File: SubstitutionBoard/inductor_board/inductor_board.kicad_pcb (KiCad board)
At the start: 2 copper layers, 275.5 x 89.4 mm, 220 parts, among them J1 Conn_Coaxial_Power, J2 Barrel_Jack_Switch, J3 Conn_01x18, J4 Conn_01x06_Socket, K1 FINDER-32.21-x000, K10 FINDER-32.21-x000, K11 FINDER-32.21-x000, K12 FINDER-32.21-x000, K13 FINDER-32.21-x000, K14 FINDER-32.21-x000, K15 FINDER-32.21-x000, K16 FINDER-32.21-x000, K2 FINDER-32.21-x000, K3 FINDER-32.21-x000, K4 FINDER-32.21-x000, K5 FINDER-32.21-x000, K6 FINDER-32.21-x000, K7 FINDER-32.21-x000, K8 FINDER-32.21-x000, K9 FINDER-32.21-x000, SW1 SW_DIP_x08, SW2 SW_DIP_x08, U1 TLP175A, U10 LM317_SOT-223, U11 TLP175A, U12 LM317_SOT-223, U13 TLP175A, U14 LM317_SOT-223, U15 TLP175A, U16 LM317_SOT-223, U17 TLP175A, U18 LM317_SOT-223, U19 TLP175A, U2 LM317_SOT-223, U20 LM317_SOT-223, U21 TLP175A, U22 LM317_SOT-223, U23 TLP175A, U24 LM317_SOT-223, U25 TLP175A, U26 LM317_SOT-223, U27 TLP175A, U28 LM317_SOT-223, U29 TLP175A, U3 TLP175A, U30 LM317_SOT-223, U31 TLP175A, U32 LM317_SOT-223, U33 L7805, U4 LM317_SOT-223, U5 TLP175A, U6 LM317_SOT-223, U7 TLP175A, U8 LM317_SOT-223, U9 TLP175A

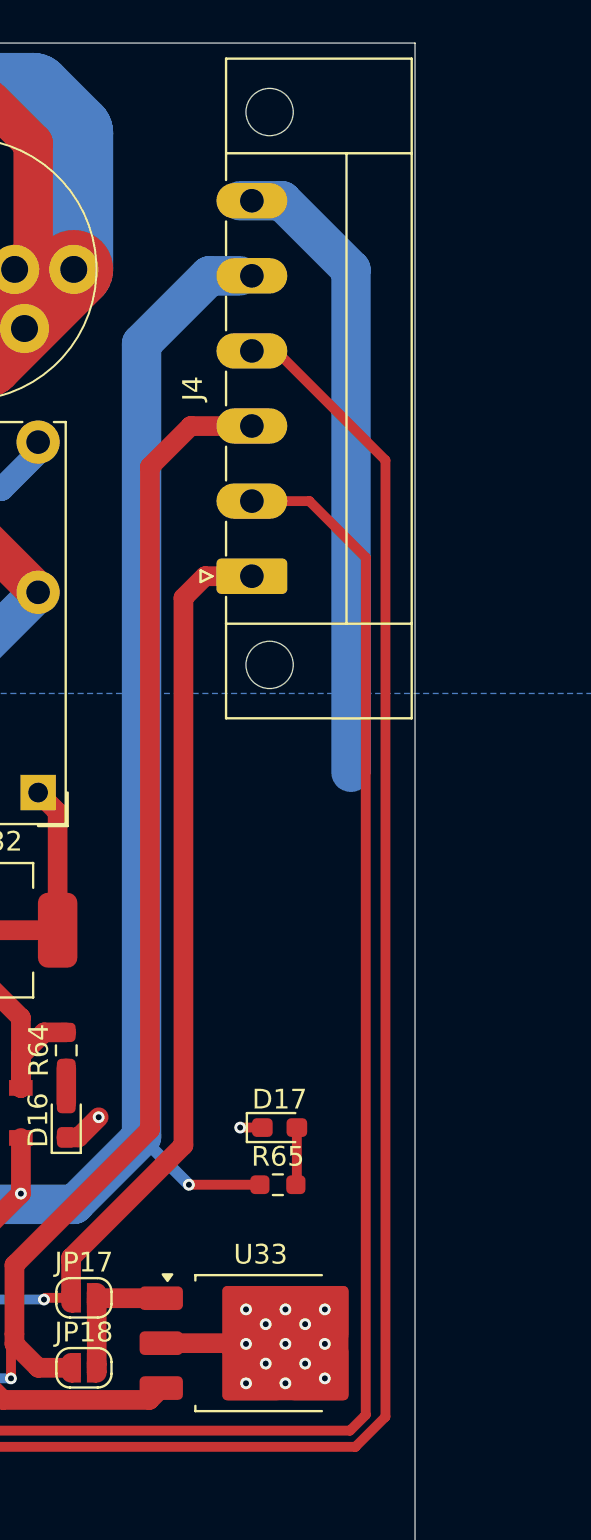
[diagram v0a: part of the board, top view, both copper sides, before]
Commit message: Update inductor_board.kicad_pcb
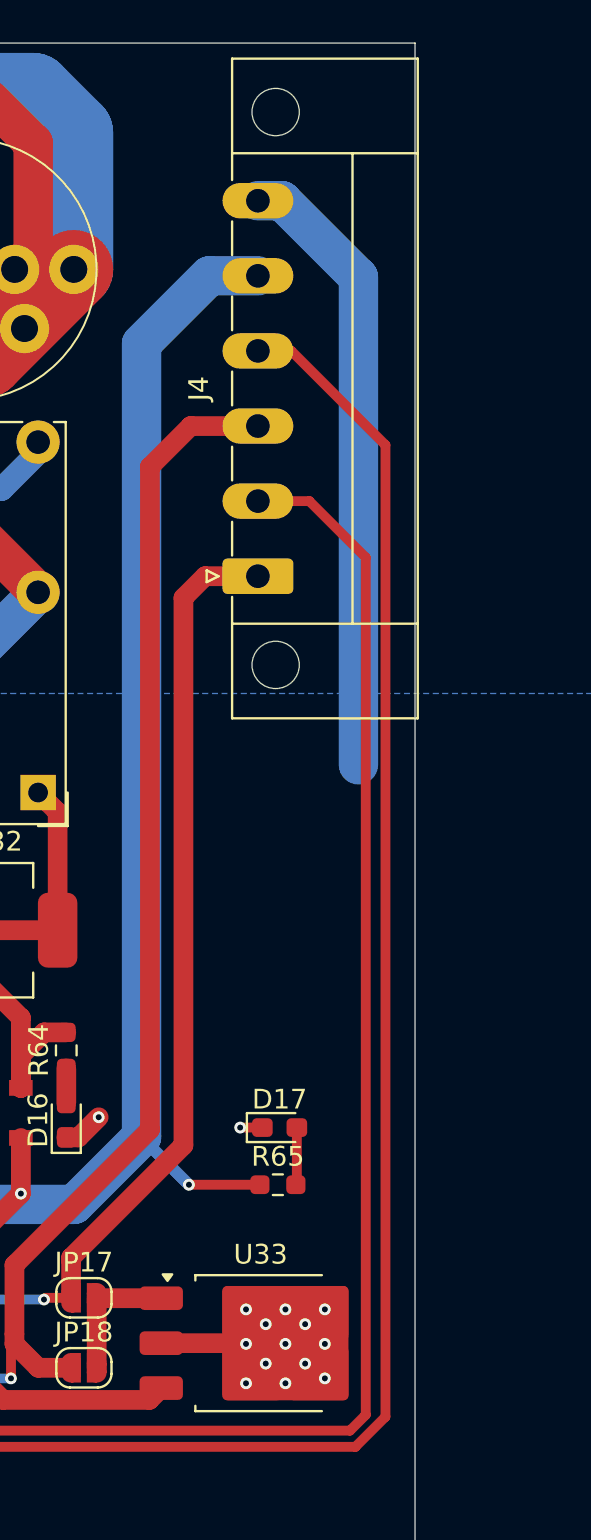
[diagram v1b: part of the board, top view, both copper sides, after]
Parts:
- moved J4 0.31 mm to (477.7, 185.1)
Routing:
- net GND: track 242.6 -> 241.5 mm
- net +5V: track 496.5 -> 497.4 mm
- net -24V: track 293.1 -> 292.2 mm
- net +24V: track 272.1 -> 273.0 mm
- net +12V: track 280.3 -> 281.3 mm
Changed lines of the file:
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@@
 	(footprint "Connector_Phoenix_MC:PhoenixContact_MC_1,5_6-GF-3.81_1x06_P3.81mm_Horizontal_ThreadedFlange_MountHole"
 		(layer "F.Cu")
-		(at 477.393 185.1255 90)
+		(at 477.7 185.1255 90)
 		(descr "Generic Phoenix Contact connector footprint for: MC_1,5/6-GF-3.81; number of pins: 06; pin pitch: 3.81mm; Angled; threaded flange; footprint includes mount hole for mounting screw: ISO 1481-ST 2.2x4.5 C or ISO 7049-ST 2.2x4.5 C (http://www.fasteners.eu/standards/ISO/7049/) || order number: 1827907 8A 160V")
 		(tags "phoenix_contact connector MC_01x06_GF_3.81mm_MH")
@@
 	)
 	(segment
-		(start 476.79624 166.0755)
-		(end 478.92124 166.0755)
+		(start 482.8 169.95426)
+		(end 482.8 194.69674)
 		(width 2)
 		(layer "B.Cu")
@@
 	(segment
 		(start 478.92124 166.0755)
-		(end 482.42124 169.5755)
+		(end 482.8 169.95426)
 		(width 2)
 		(layer "B.Cu")
@@
 	)
 	(segment
-		(start 482.42124 169.5755)
-		(end 482.42124 195.0755)
+		(start 477.7 166.0755)
+		(end 478.92124 166.0755)
 		(width 2)
 		(layer "B.Cu")
@@
 	)
 	(segment
-		(start 471.79624 173.3255)
-		(end 475.23624 169.8855)
+		(start 229.48374 188.388)
+		(end 229.54624 188.4505)
 		(width 2)
 		(layer "B.Cu")
@@
 	)
 	(segment
-		(start 229.48374 188.388)
-		(end 229.54624 188.4505)
+		(start 471.79624 173.3255)
+		(end 475.23624 169.8855)
 		(width 2)
 		(layer "B.Cu")
@@
 	)
 	(segment
-		(start 475.23624 169.8855)
-		(end 476.79624 169.8855)
-		(width 2)
-		(layer "B.Cu")
-		(net 131)
-	)
-	(segment
 		(start 471.79624 213.5755)
 		(end 471.79624 213.59624)
@@
 	)
 	(segment
-		(start 471.79624 213.5755)
-		(end 471.79624 173.3255)
+		(start 475.23624 169.8855)
+		(end 477.7 169.8855)
 		(width 2)
 		(layer "B.Cu")
@@
 	)
 	(segment
+		(start 471.79624 213.5755)
+		(end 471.79624 173.3255)
+		(width 2)
+		(layer "B.Cu")
+		(net 131)
+	)
+	(segment
 		(start 223.83624 194.0355)
 		(end 229.48374 188.388)
@@
 	)
 	(segment
-		(start 468.22124 219.8255)
-		(end 468.22124 219.7005)
-		(width 1)
-		(layer "F.Cu")
-		(net 144)
-	)
-	(segment
 		(start 260.63124 236.7755)
 		(end 256.83124 240.5755)
@@
 	)
 	(segment
+		(start 475.02124 185.1255)
+		(end 477.7 185.1255)
+		(width 1)
+		(layer "F.Cu")
+		(net 144)
+	)
+	(segment
 		(start 466.93374 221.738)
 		(end 466.84624 221.8255)
@@
 	)
 	(segment
-		(start 473.92124 186.2255)
-		(end 475.02124 185.1255)
+		(start 468.22124 219.8255)
+		(end 468.22124 219.7005)
 		(width 1)
 		(layer "F.Cu")
@@
 	)
 	(segment
-		(start 475.02124 185.1255)
-		(end 476.79624 185.1255)
+		(start 468.22124 219.7005)
+		(end 473.92124 214.0005)
 		(width 1)
 		(layer "F.Cu")
@@
 	)
 	(segment
-		(start 468.22124 219.7005)
-		(end 473.92124 214.0005)
+		(start 473.92124 186.2255)
+		(end 475.02124 185.1255)
 		(width 1)
 		(layer "F.Cu")
@@
 	)
 	(segment
-		(start 271.09674 228.6)
-		(end 460.686689 228.6)
+		(start 460.686689 228.6)
+		(end 460.811189 228.4755)
 		(width 0.5)
 		(layer "F.Cu")
@@
 	)
 	(segment
-		(start 257.44624 242.4505)
-		(end 256.49624 242.4505)
+		(start 482.37124 228.4755)
+		(end 483.17124 227.6755)
 		(width 0.5)
 		(layer "F.Cu")
@@
 	)
 	(segment
-		(start 460.686689 228.6)
-		(end 460.811189 228.4755)
+		(start 460.811189 228.4755)
+		(end 482.37124 228.4755)
 		(width 0.5)
 		(layer "F.Cu")
@@
 	)
 	(segment
-		(start 482.37124 228.4755)
-		(end 483.17124 227.6755)
+		(start 257.44624 242.4505)
+		(end 256.49624 242.4505)
 		(width 0.5)
 		(layer "F.Cu")
@@
 	)
 	(segment
-		(start 480.31124 181.3155)
-		(end 476.79624 181.3155)
+		(start 483.17124 184.1755)
+		(end 480.31124 181.3155)
 		(width 0.5)
 		(layer "F.Cu")
@@
 	)
 	(segment
-		(start 483.17124 227.6755)
-		(end 483.17124 184.1755)
+		(start 257.34624 242.3505)
+		(end 271.09674 228.6)
 		(width 0.5)
 		(layer "F.Cu")
@@
 	)
 	(segment
-		(start 257.34624 242.3505)
-		(end 271.09674 228.6)
+		(start 256.83124 242.8655)
+		(end 257.34624 242.3505)
 		(width 0.5)
 		(layer "F.Cu")
@@
 	)
 	(segment
-		(start 256.83124 242.8655)
-		(end 257.34624 242.3505)
+		(start 256.49624 242.4505)
+		(end 255.93124 243.0155)
 		(width 0.5)
 		(layer "F.Cu")
@@
 	)
 	(segment
-		(start 460.811189 228.4755)
-		(end 482.37124 228.4755)
+		(start 480.31124 181.3155)
+		(end 477.7 181.3155)
 		(width 0.5)
 		(layer "F.Cu")
@@
 	)
 	(segment
-		(start 256.49624 242.4505)
-		(end 255.93124 243.0155)
+		(start 271.09674 228.6)
+		(end 460.686689 228.6)
+		(width 0.5)
+		(layer "F.Cu")
+		(net 182)
+	)
+	(segment
+		(start 483.17124 227.6755)
+		(end 483.17124 184.1755)
 		(width 0.5)
 		(layer "F.Cu")
@@
 	)
 	(segment
-		(start 483.17124 184.1755)
-		(end 480.31124 181.3155)
+		(start 272.44674 229.3)
+		(end 482.64674 229.3)
 		(width 0.5)
 		(layer "F.Cu")
-		(net 182)
+		(net 191)
 	)
 	(segment
-		(start 484.17124 179.24424)
-		(end 478.6225 173.6955)
+		(start 484.17124 227.7755)
+		(end 484.17124 178.47124)
+		(width 0.5)
+		(layer "F.Cu")
+		(net 191)
+	)
+	(segment
+		(start 482.64674 229.3)
+		(end 484.17124 227.7755)
 		(width 0.5)
 		(layer "F.Cu")
@@
 	)
 	(segment
-		(start 484.17124 227.7755)
-		(end 484.17124 179.24424)
+		(start 484.17124 178.47124)
+		(end 479.3955 173.6955)
 		(width 0.5)
 		(layer "F.Cu")
@@
 	)
 	(segment
-		(start 478.6225 173.6955)
-		(end 476.79624 173.6955)
-		(width 0.5)
-		(layer "F.Cu")
-		(net 191)
-	)
-	(segment
 		(start 258.83124 245.2355)
 		(end 258.83124 242.9155)
@@
 	)
 	(segment
-		(start 272.44674 229.3)
-		(end 482.64674 229.3)
-		(width 0.5)
-		(layer "F.Cu")
-		(net 191)
-	)
-	(segment
-		(start 482.64674 229.3)
-		(end 484.17124 227.7755)
+		(start 479.3955 173.6955)
+		(end 477.7 173.6955)
 		(width 0.5)
 		(layer "F.Cu")
@@
 	)
 	(segment
-		(start 466.55874 225.288)
-		(end 465.34624 224.0755)
+		(start 465.34624 220.0755)
+		(end 472.22124 213.2005)
 		(width 1)
 		(layer "F.Cu")
@@
 	)
 	(segment
-		(start 465.34624 220.0755)
-		(end 472.22124 213.2005)
+		(start 474.29124 177.5055)
+		(end 477.7 177.5055)
 		(width 1)
 		(layer "F.Cu")
@@
 	)
 	(segment
-		(start 472.22124 179.5755)
-		(end 474.29124 177.5055)
+		(start 466.55874 225.288)
+		(end 465.34624 224.0755)
 		(width 1)
 		(layer "F.Cu")
@@
 	)
 	(segment
-		(start 474.29124 177.5055)
-		(end 476.79624 177.5055)
+		(start 465.34624 223.5755)
+		(end 465.34624 220.0755)
 		(width 1)
 		(layer "F.Cu")
@@
 	)
 	(segment
-		(start 472.22124 213.2005)
-		(end 472.22124 179.5755)
-		(width 1)
-		(layer "F.Cu")
-		(net 216)
-	)
-	(segment
-		(start 465.34624 223.5755)
-		(end 465.34624 220.0755)
+		(start 472.22124 179.5755)
+		(end 474.29124 177.5055)
 		(width 1)
 		(layer "F.Cu")
@@
 		(layer "F.Cu")
 		(net 216)
+	)
+	(segment
+		(start 472.22124 213.2005)
+		(end 472.22124 179.5755)
+		(width 1)
+		(layer "F.Cu")
+		(net 216)
